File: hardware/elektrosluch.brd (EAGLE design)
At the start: 38.7 x 121.6 mm, 30 parts, among them IC1 OPA2134UA, X1 STEREOJACK, X2 STEREOJACK

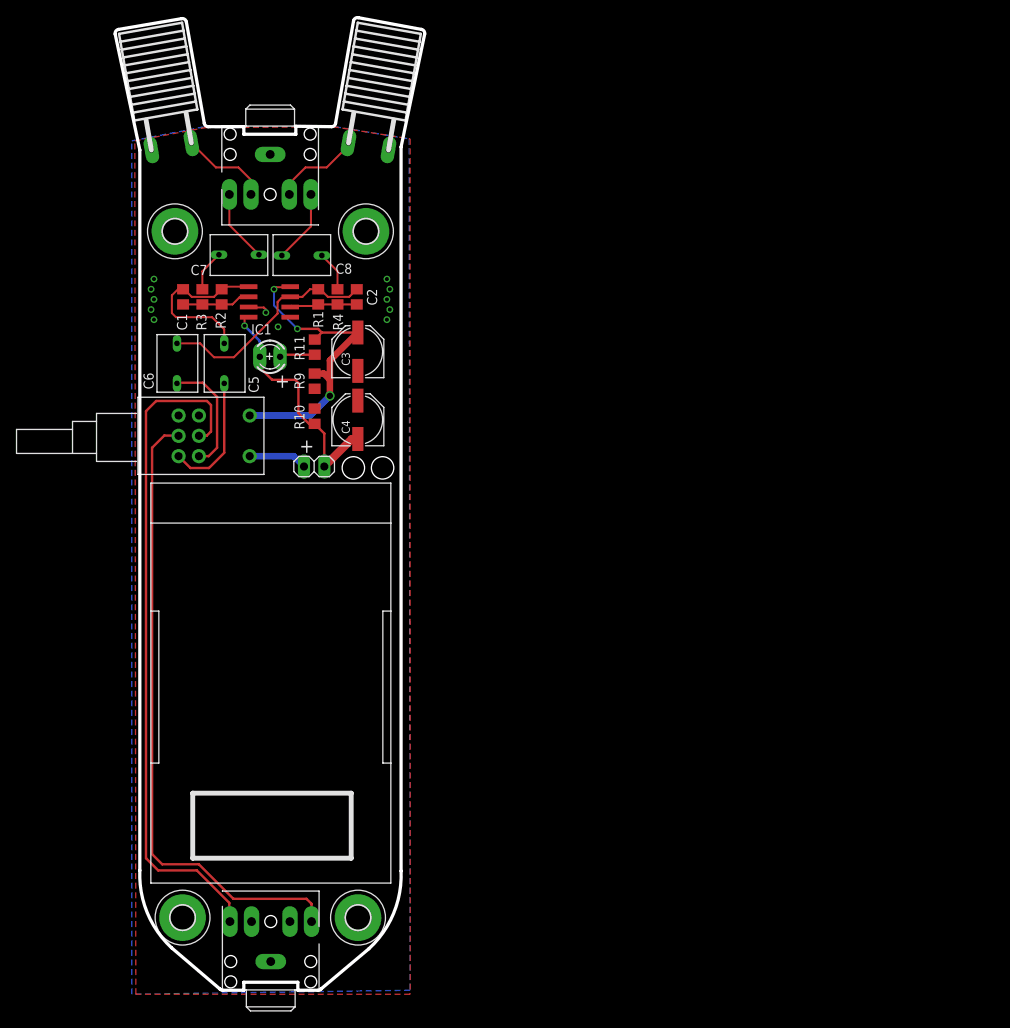
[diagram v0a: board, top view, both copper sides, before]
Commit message: Layout tests
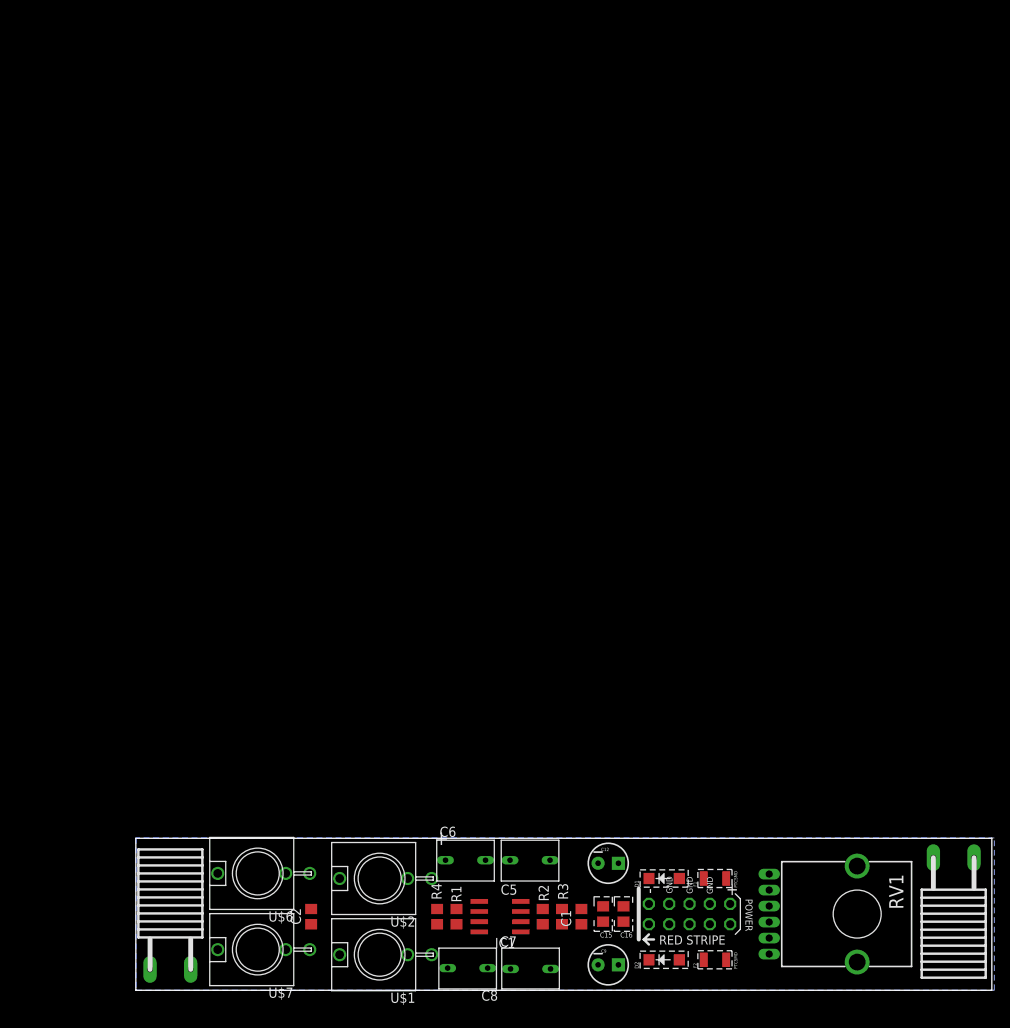
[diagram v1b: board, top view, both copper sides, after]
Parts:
- removed ALPS_POT: RK0971221Z05, audio-pots:ALPS_RK0971221Z0X
- removed C3, C4: 220uF, rcl:PANASONIC_D
- removed H1, H2, H3, H4: MOUNT-PAD-ROUND3.0, holes:3,0-PAD
- removed JP1: (no value), pinhead:1X02
- removed LED1: LED, mojakniznica:LED3MM
- removed R10, R9: 100k, rcl:R0805
- removed R11: 1k, rcl:R0805
- removed U$3: (no value), mojakniznica:ELEKTROSLUCH3
- removed U$4: (no value), mojakniznica:LOM_BACK
- removed X1, X2: STEREOJACK, adafruit:STX3100
- added C12, C9: 220uf, SparkFun-Passives:CPOL-RADIAL-10UF-25V
- added C15, C16: 100n, TomW:R0805
- added D1, D2: (no value), diode:SOD123
- added F1, F2: PTCSMD, SparkFun-PowerIC:PTC-1206
- added POWER: (no value), TomW:MA05-2
- added RV1: (no value), SparkFun-Electromechanical:POT_PANASONIC_DUAL_VERT_KIT
- added U$1, U$6, U$7: THONKICONNNEW, MusicThingModular:WQP-PJ301M-12_JACK
- U$2: value BATT -> THONKICONNNEW; device mojakniznica:BATT -> MusicThingModular:WQP-PJ301M-12_JACK
- moved INDUCTOR_1 132.2 mm to (102.2, 16.6), turned to 180 degrees
- moved INDUCTOR_2 105.8 mm to (4.32, 2.60), turned to 0 degrees
- moved C7 96.4 mm to (49.3, 2.67), turned to 0 degrees
- moved C1 92.1 mm to (55.7, 9.21), turned to 90 degrees
- moved C8 91.5 mm to (41.5, 2.77), turned to 180 degrees
- moved R3 89.6 mm to (53.3, 9.21), turned to 270 degrees
- moved R2 87.2 mm to (50.9, 9.21), turned to 90 degrees
- moved IC1 82.1 mm to (45.5, 9.21), turned to 90 degrees
- moved R1 79.4 mm to (40.1, 9.21), turned to 90 degrees
- moved R4 78.5 mm to (37.7, 9.21), turned to 270 degrees
- moved C2 77.7 mm to (21.9, 9.21), turned to 90 degrees
- moved C5 72.9 mm to (49.3, 16.3), turned to 180 degrees
- moved C6 71.8 mm to (41.2, 16.3), turned to 180 degrees
- moved U$2 1.51 mm to (30.5, 14.0)
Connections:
- removed net +5V: ALPS_POT.S1, C3.+, IC1.8, R11.2, R9.2
- removed net -5V: C4.-, IC1.4, JP1.1, LED1.K, R10.1
- new net +12V: C15.2, C9.1, D2.C, F1.1, IC1.8
- new net -12V: C12.2, C16.1, D1.A, F2.1, IC1.4
- net GND: now also C12.1, C15.1, C16.2, C9.2, D1.C, D2.A, POWER.3, POWER.4, POWER.5, POWER.6, POWER.7, POWER.8, RV1.A3, RV1.B3, U$1.P$1_TIP, U$2.P$1_TIP, U$6.P$3_SLEEVE, U$7.P$3_SLEEVE; no longer ALPS_POT.G1, ALPS_POT.G2, C3.-, C4.+, H1.B3,0, H2.B3,0, H3.B3,0, H4.B3,0, R10.2, R9.1, X1.1, X2.1
- net N$10: now also U$2.P$2_SWITCH; no longer X1.2
- net N$12: now also U$1.P$2_SWITCH; no longer X1.4
- net N$13: now also U$2.P$3_SLEEVE; no longer X1.3
- net N$14: now also F1.2, POWER.10, POWER.9; no longer LED1.A, R11.1
- net N$16: now also F2.2, POWER.1, POWER.2; no longer ALPS_POT.S2, JP1.2
- net N$3: now also RV1.A1; no longer ALPS_POT.I1
- net N$6: now also RV1.B1; no longer ALPS_POT.I2
- net N$7: now also RV1.A2, U$6.P$1_TIP; no longer ALPS_POT.O1, X2.5
- net N$8: now also U$1.P$3_SLEEVE; no longer X1.5
- net N$9: now also RV1.B2, U$7.P$1_TIP; no longer ALPS_POT.O2, X2.2
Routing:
- net N$9: track 85.8 -> 0.00 mm
- net N$7: track 79.5 -> 0.00 mm
- net +5V: track 40.2 -> 0.00 mm, vias 3 -> 0
- net -5V: track 30.6 -> 0.00 mm, vias 1 -> 0
- net N$5: track 28.4 -> 0.00 mm
- net N$2: track 22.2 -> 0.00 mm
- net N$3: track 15.8 -> 0.00 mm
- net N$6: track 14.9 -> 0.00 mm
- net N$13: track 11.4 -> 0.00 mm
- net N$12: track 11.2 -> 0.00 mm
- net N$10: track 9.14 -> 0.00 mm
- net N$8: track 9.06 -> 0.00 mm
- net N$1: track 8.59 -> 0.00 mm
- net N$4: track 8.45 -> 0.00 mm
- net N$16: track 7.32 -> 0.00 mm
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- removed copper zone on layer 1, net GND
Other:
- board size 38.7 x 121.6 mm -> 107 x 19 mm
